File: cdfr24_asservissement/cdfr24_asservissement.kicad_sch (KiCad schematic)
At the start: 60 parts, among them J1 Connecteur batterie, J10 Free Connecteur, J11 Conn_01x02, J12 Conn_01x02, J13 Connecteur Odométrie, J14 Conn_ST_STDC14, J2 Conn_01x03, J3 Conn_01x05, J4 Connecteur Programmation, J5 Conn_01x03, J6 Connecteur Odométrie, J7 Conn_01x03, Q13 Q_NMOS_GDS, U1 LM317_SOT-223, U3 STM32F401RCTx, U4 LMR16020PDDA, U4 LSM6DSL, Y1 Crystal_GND24

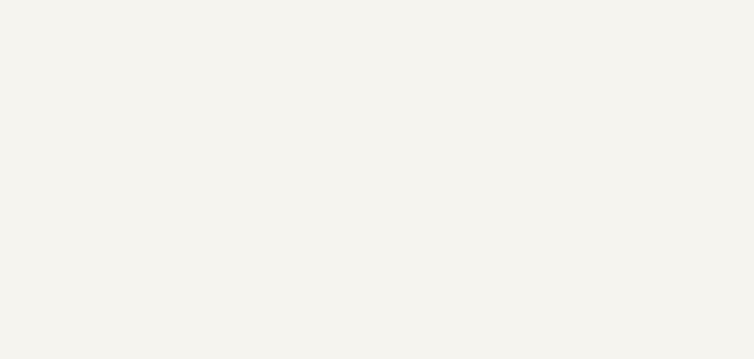
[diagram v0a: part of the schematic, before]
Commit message: Resolve some errors
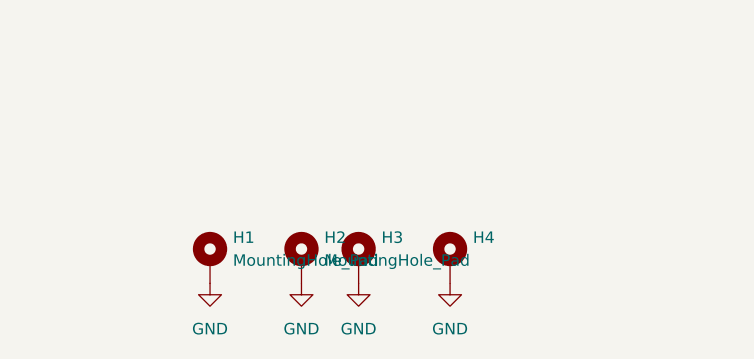
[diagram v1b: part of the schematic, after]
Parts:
- added H1, H2, H3, H4: MountingHole_Pad, MountingHole:MountingHole_3.2mm_M3_Pad_Via, symbol Mechanical:MountingHole_Pad
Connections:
- net GND: now also H1.1, H2.1, H3.1, H4.1
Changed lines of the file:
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@@
+    )
+  )
+  (symbol (lib_id "power:GND") (at 45.72 391.16 0) (unit 1)
+    (in_bom yes) (on_board yes) (dnp no) (fields_autoplaced)
+    (property "Reference" "#PWR078" (at 45.72 397.51 0)
+      (effects (font (size 1.27 1.27)) hide)
+    )
+    (property "Value" "GND" (at 45.72 396.24 0)
+      (effects (font (size 1.27 1.27)))
+    )
+    (property "Footprint" "" (at 45.72 391.16 0)
+      (effects (font (size 1.27 1.27)) hide)
+    )
+    (property "Datasheet" "" (at 45.72 391.16 0)
+      (effects (font (size 1.27 1.27)) hide)
+    )
+    (pin "1")
+    (instances
+      (project "Asservissement_CDFR_2023"
+        (path "/aba37299-4f54-471d-ab35-d760532fd54c"
+          (reference "#PWR078") (unit 1)
+        )
+      )
+      (project "cdfr24_asservissement"
+        (path "/c6b82269-16f5-49e6-8b51-4d12a40a3077"
+          (reference "#PWR077") (unit 1)
+        )
+      )
     )
   )
@@
     )
   )
+  (symbol (lib_id "power:GND") (at 55.88 391.16 0) (unit 1)
+    (in_bom yes) (on_board yes) (dnp no) (fields_autoplaced)
+    (property "Reference" "#PWR079" (at 55.88 397.51 0)
+      (effects (font (size 1.27 1.27)) hide)
+    )
+    (property "Value" "GND" (at 55.88 396.24 0)
+      (effects (font (size 1.27 1.27)))
+    )
+    (property "Footprint" "" (at 55.88 391.16 0)
+      (effects (font (size 1.27 1.27)) hide)
+    )
+    (property "Datasheet" "" (at 55.88 391.16 0)
+      (effects (font (size 1.27 1.27)) hide)
+    )
+    (pin "1")
+    (instances
+      (project "Asservissement_CDFR_2023"
+        (path "/aba37299-4f54-471d-ab35-d760532fd54c"
+          (reference "#PWR079") (unit 1)
+        )
+      )
+      (project "cdfr24_asservissement"
+        (path "/c6b82269-16f5-49e6-8b51-4d12a40a3077"
+          (reference "#PWR078") (unit 1)
+        )
+      )
+    )
+  )
   (symbol (lib_id "Regulator_Linear:LM317_SOT-223") (at 219.075 38.735 0) (unit 1)
     (in_bom yes) (on_board yes) (dnp no) (fields_autoplaced)
@@
         (path "/c6b82269-16f5-49e6-8b51-4d12a40a3077"
           (reference "C11") (unit 1)
+        )
+      )
+    )
+  )
+  (symbol (lib_id "Mechanical:MountingHole_Pad") (at 29.21 388.62 0) (unit 1)
+    (in_bom yes) (on_board yes) (dnp no) (fields_autoplaced)
+    (property "Reference" "H1" (at 31.75 386.0799 0)
+      (effects (font (size 1.27 1.27)) (justify left))
+    )
+    (property "Value" "MountingHole_Pad" (at 31.75 388.6199 0)
+      (effects (font (size 1.27 1.27)) (justify left))
+    )
+    (property "Footprint" "MountingHole:MountingHole_3.2mm_M3_Pad_Via" (at 29.21 388.62 0)
+      (effects (font (size 1.27 1.27)) hide)
+    )
+    (property "Datasheet" "~" (at 29.21 388.62 0)
+      (effects (font (size 1.27 1.27)) hide)
+    )
+    (pin "1")
+    (instances
+      (project "Asservissement_CDFR_2023"
+        (path "/aba37299-4f54-471d-ab35-d760532fd54c"
+          (reference "H1") (unit 1)
+        )
+      )
+      (project "cdfr24_asservissement"
+        (path "/c6b82269-16f5-49e6-8b51-4d12a40a3077"
+          (reference "H1") (unit 1)
         )
       )
@@
     )
   )
+  (symbol (lib_id "Mechanical:MountingHole_Pad") (at 39.37 388.62 0) (unit 1)
+    (in_bom yes) (on_board yes) (dnp no) (fields_autoplaced)
+    (property "Reference" "H2" (at 41.91 386.0799 0)
+      (effects (font (size 1.27 1.27)) (justify left))
+    )
+    (property "Value" "MountingHole_Pad" (at 41.91 388.6199 0)
+      (effects (font (size 1.27 1.27)) (justify left))
+    )
+    (property "Footprint" "MountingHole:MountingHole_3.2mm_M3_Pad_Via" (at 39.37 388.62 0)
+      (effects (font (size 1.27 1.27)) hide)
+    )
+    (property "Datasheet" "~" (at 39.37 388.62 0)
+      (effects (font (size 1.27 1.27)) hide)
+    )
+    (pin "1")
+    (instances
+      (project "Asservissement_CDFR_2023"
+        (path "/aba37299-4f54-471d-ab35-d760532fd54c"
+          (reference "H2") (unit 1)
+        )
+      )
+      (project "cdfr24_asservissement"
+        (path "/c6b82269-16f5-49e6-8b51-4d12a40a3077"
+          (reference "H2") (unit 1)
+        )
+      )
+    )
+  )
   (symbol (lib_id "Connector_Generic:Conn_01x02") (at 71.755 331.47 90) (mirror x) (unit 1)
     (in_bom yes) (on_board yes) (dnp no) (fields_autoplaced)
@@
     )
   )
+  (symbol (lib_id "Mechanical:MountingHole_Pad") (at 45.72 388.62 0) (unit 1)
+    (in_bom yes) (on_board yes) (dnp no) (fields_autoplaced)
+    (property "Reference" "H3" (at 48.26 386.0799 0)
+      (effects (font (size 1.27 1.27)) (justify left))
+    )
+    (property "Value" "MountingHole_Pad" (at 48.26 388.6199 0)
+      (effects (font (size 1.27 1.27)) (justify left) hide)
+    )
+    (property "Footprint" "MountingHole:MountingHole_3.2mm_M3_Pad_Via" (at 45.72 388.62 0)
+      (effects (font (size 1.27 1.27)) hide)
+    )
+    (property "Datasheet" "~" (at 45.72 388.62 0)
+      (effects (font (size 1.27 1.27)) hide)
+    )
+    (pin "1")
+    (instances
+      (project "Asservissement_CDFR_2023"
+        (path "/aba37299-4f54-471d-ab35-d760532fd54c"
+          (reference "H3") (unit 1)
+        )
+      )
+      (project "cdfr24_asservissement"
+        (path "/c6b82269-16f5-49e6-8b51-4d12a40a3077"
+          (reference "H3") (unit 1)
+        )
+      )
+    )
+  )
   (symbol (lib_id "Connector_Generic:Conn_01x05") (at 398.526 75.438 270) (mirror x) (unit 1)
     (in_bom yes) (on_board yes) (dnp no) (fields_autoplaced)
@@
     )
   )
+  (symbol (lib_id "Mechanical:MountingHole_Pad") (at 55.88 388.62 0) (unit 1)
+    (in_bom yes) (on_board yes) (dnp no) (fields_autoplaced)
+    (property "Reference" "H4" (at 58.42 386.0799 0)
+      (effects (font (size 1.27 1.27)) (justify left))
+    )
+    (property "Value" "MountingHole_Pad" (at 58.42 388.6199 0)
+      (effects (font (size 1.27 1.27)) (justify left) hide)
+    )
+    (property "Footprint" "MountingHole:MountingHole_3.2mm_M3_Pad_Via" (at 55.88 388.62 0)
+      (effects (font (size 1.27 1.27)) hide)
+    )
+    (property "Datasheet" "~" (at 55.88 388.62 0)
+      (effects (font (size 1.27 1.27)) hide)
+    )
+    (pin "1")
+    (instances
+      (project "Asservissement_CDFR_2023"
+        (path "/aba37299-4f54-471d-ab35-d760532fd54c"
+          (reference "H4") (unit 1)
+        )
+      )
+      (project "cdfr24_asservissement"
+        (path "/c6b82269-16f5-49e6-8b51-4d12a40a3077"
+          (reference "H4") (unit 1)
+        )
+      )
+    )
+  )
   (symbol (lib_id "Device:R") (at 119.38 248.92 90) (unit 1)
     (in_bom yes) (on_board yes) (dnp no) (fields_autoplaced)
@@
     )
   )
+  (symbol (lib_id "power:GND") (at 39.37 391.16 0) (unit 1)
+    (in_bom yes) (on_board yes) (dnp no) (fields_autoplaced)
+    (property "Reference" "#PWR077" (at 39.37 397.51 0)
+      (effects (font (size 1.27 1.27)) hide)
+    )
+    (property "Value" "GND" (at 39.37 396.24 0)
+      (effects (font (size 1.27 1.27)))
+    )
+    (property "Footprint" "" (at 39.37 391.16 0)
+      (effects (font (size 1.27 1.27)) hide)
+    )
+    (property "Datasheet" "" (at 39.37 391.16 0)
+      (effects (font (size 1.27 1.27)) hide)
+    )
+    (pin "1")
+    (instances
+      (project "Asservissement_CDFR_2023"
+        (path "/aba37299-4f54-471d-ab35-d760532fd54c"
+          (reference "#PWR077") (unit 1)
+        )
+      )
+      (project "cdfr24_asservissement"
+        (path "/c6b82269-16f5-49e6-8b51-4d12a40a3077"
+          (reference "#PWR076") (unit 1)
+        )
+      )
+    )
+  )
   (symbol (lib_id "power:GND") (at 113.03 248.92 270) (unit 1)
     (in_bom yes) (on_board yes) (dnp no)
@@
         )
       )
+    )
+  )
+  (symbol (lib_id "power:GND") (at 29.21 391.16 0) (unit 1)
+    (in_bom yes) (on_board yes) (dnp no) (fields_autoplaced)
+    (property "Reference" "#PWR02" (at 29.21 397.51 0)
+      (effects (font (size 1.27 1.27)) hide)
+    )
+    (property "Value" "GND" (at 29.21 396.24 0)
+      (effects (font (size 1.27 1.27)))
+    )
+    (property "Footprint" "" (at 29.21 391.16 0)
+      (effects (font (size 1.27 1.27)) hide)
+    )
+    (property "Datasheet" "" (at 29.21 391.16 0)
+      (effects (font (size 1.27 1.27)) hide)
+    )
+    (pin "1")
+    (instances
+      (project "Asservissement_CDFR_2023"
+        (path "/aba37299-4f54-471d-ab35-d760532fd54c"
+          (reference "#PWR02") (unit 1)
+        )
+      )
+      (project "cdfr24_asservissement"
+        (path "/c6b82269-16f5-49e6-8b51-4d12a40a3077"
+          (reference "#PWR075") (unit 1)
+        )
+      )
